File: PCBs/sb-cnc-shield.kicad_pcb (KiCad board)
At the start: 2 copper layers, 68.6 x 53.3 mm, 62 parts, among them P1 XMOT, P2 YMOT, P3 ZMOT, P4 AMOT, P5 UART, P6 I2C, P7 E-STOP, P8 12V-36V, SW1 RESET, U1 ARDUINO_UNO_SHIELD, U2 X, U3 Y, U4 Z, U5 A

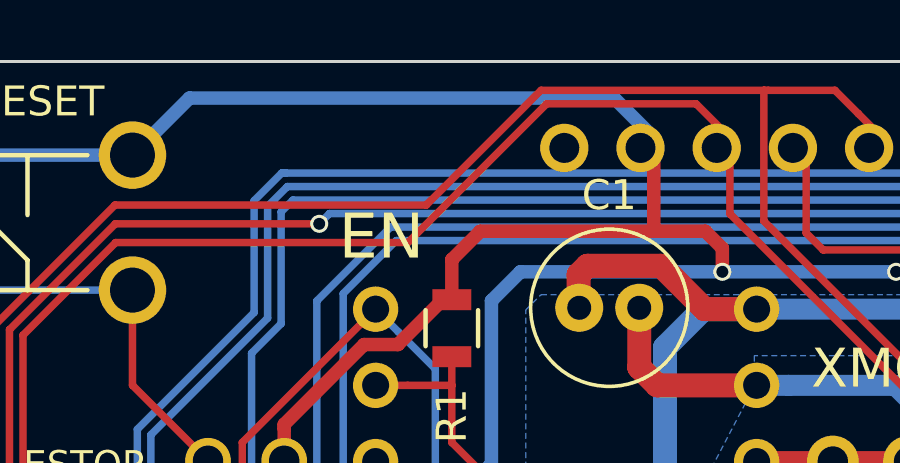
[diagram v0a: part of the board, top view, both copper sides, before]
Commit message: modify name PCBs
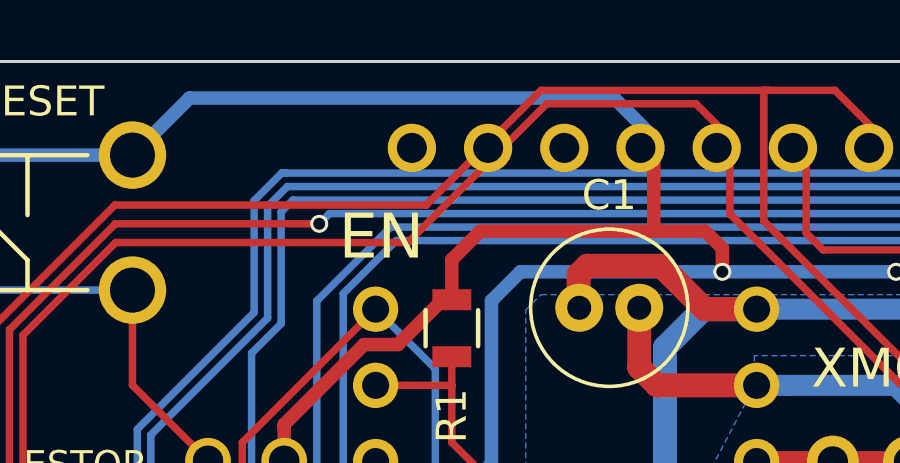
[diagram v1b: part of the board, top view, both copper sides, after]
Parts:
- P7: value E-STOP -> ES_SETUP
